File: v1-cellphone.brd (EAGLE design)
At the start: 91.4 x 44.5 mm, 75 parts, among them J1 AVRISP, J2 ZX62D-B-5P8, U1 MCP73831, U2 MEGA1284, U3 GSM_UC15, X1 BU-SMA-V, X2 16MHz, X3 CCM03-3002 R102

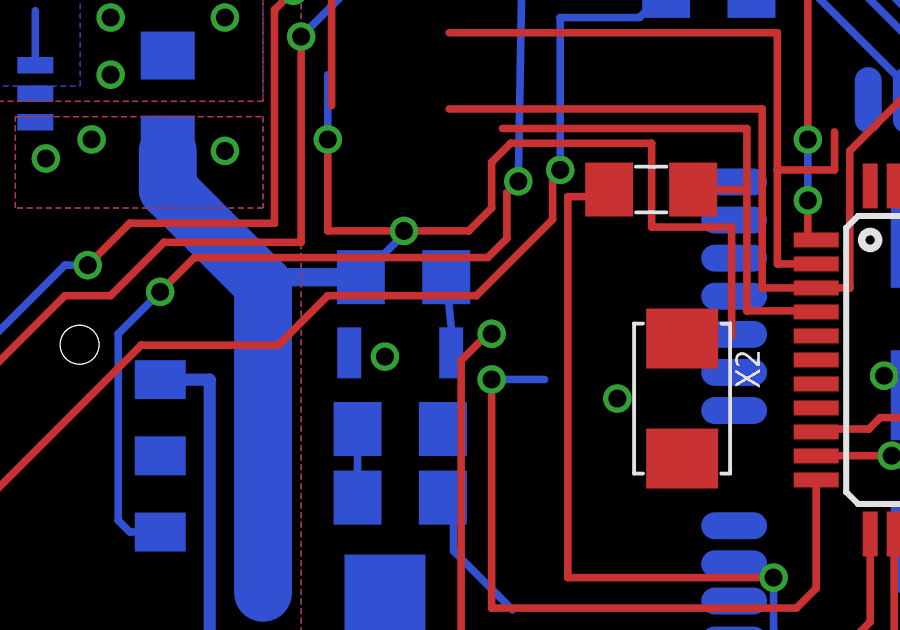
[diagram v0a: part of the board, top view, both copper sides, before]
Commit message: Added notes.
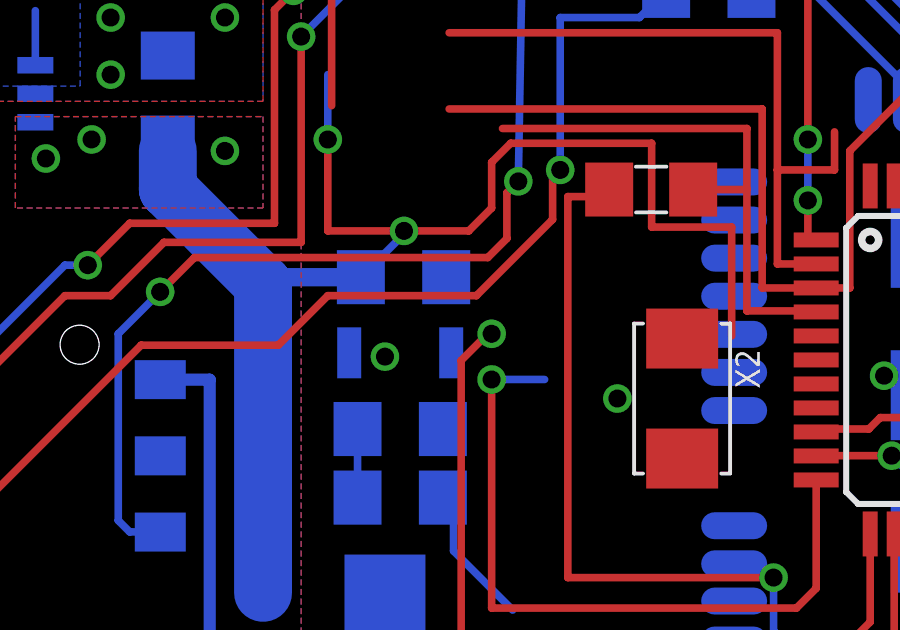
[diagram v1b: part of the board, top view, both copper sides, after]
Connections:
- net RESET renamed !RESET
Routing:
- net !RESET: track 21.0 -> 18.3 mm
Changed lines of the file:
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@@
 <wire x1="34.036" y1="36.433" x2="-52.832" y2="-61.722" width="0" layer="19" extent="1-1"/>
 </signal>
-<signal name="RESET">
-<contactref element="R4" pad="1"/>
+<signal name="!RESET">
 <contactref element="C1" pad="2"/>
 <wire x1="47.879" y1="35.671" x2="47.879" y2="33.655" width="0.254" layer="1"/>
 <wire x1="47.879" y1="33.655" x2="47.879" y2="29.591" width="0.254" layer="1"/>
 <wire x1="47.879" y1="29.591" x2="50.188" y2="29.591" width="0.254" layer="1"/>
-<wire x1="38.109" y1="28.194" x2="37.855" y2="30.715" width="0.254" layer="16"/>
-<wire x1="37.855" y1="30.715" x2="37.954" y2="30.715" width="0.254" layer="16"/>
 <wire x1="47.879" y1="35.671" x2="39.732" y2="35.671" width="0.254" layer="1"/>
 <wire x1="46.088" y1="33.636" x2="47.86" y2="33.636" width="0.254" layer="1"/>
@@
 <contactref element="S1" pad="P$2"/>
 <contactref element="U2" pad="4"/>
+<contactref element="R4" pad="1"/>
 <wire x1="38.022" y1="28.194" x2="-50.292" y2="-64.262" width="0" layer="19" extent="16-16"/>
-<wire x1="38.109" y1="28.194" x2="38.022" y2="28.194" width="0" layer="19" extent="16-16"/>
-<wire x1="39.732" y1="35.671" x2="37.954" y2="30.715" width="0" layer="19" extent="1-16"/>
+<wire x1="37.855" y1="30.715" x2="38.022" y2="28.194" width="0" layer="19" extent="16-16"/>
+<wire x1="39.732" y1="35.671" x2="37.855" y2="30.715" width="0" layer="19" extent="1-16"/>
 <wire x1="50.188" y1="29.556" x2="50.188" y2="29.591" width="0" layer="19" extent="1-1"/>
 </signal>
